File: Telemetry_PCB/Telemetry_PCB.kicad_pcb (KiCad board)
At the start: 2 copper layers, 11 parts, among them J1 Raspberry Pi Zero W, J2 Voltage Sensor, J3 Current Sensor, J4 ADC, J5 GPS

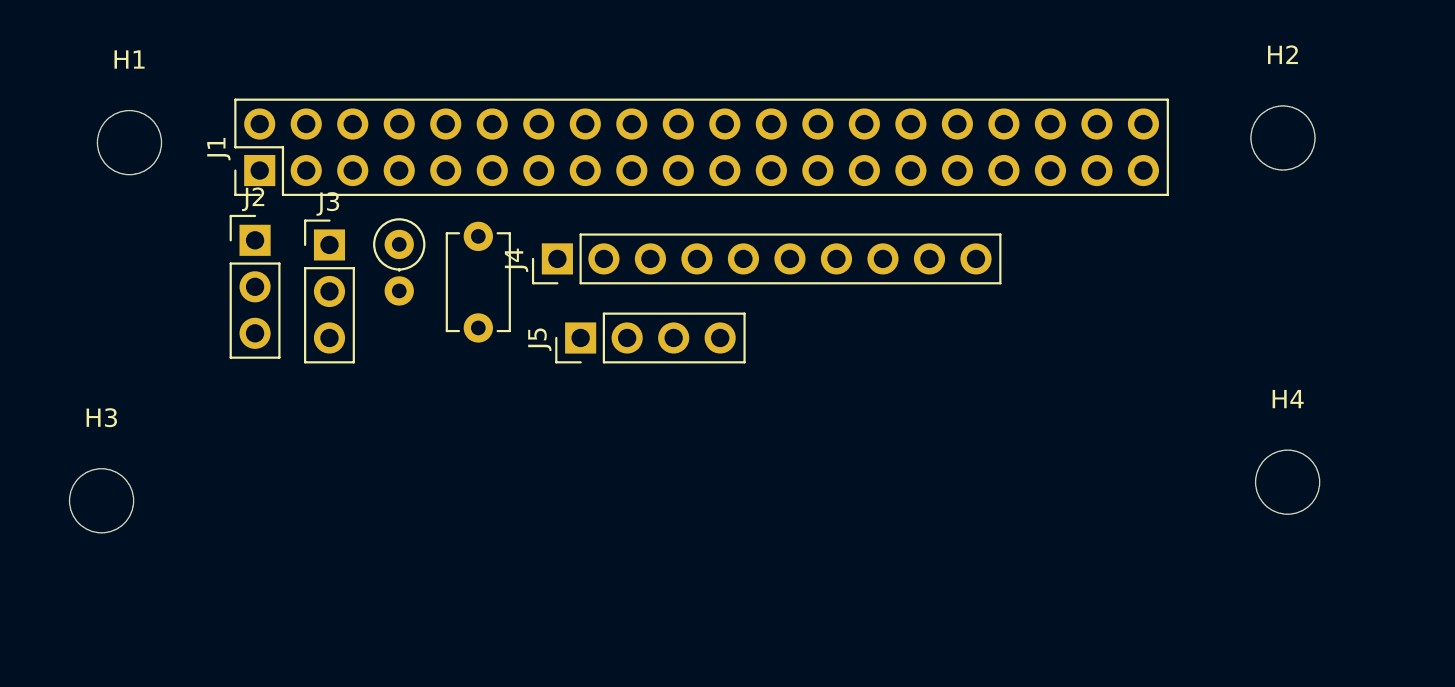
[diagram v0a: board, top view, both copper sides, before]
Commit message: Adding email system
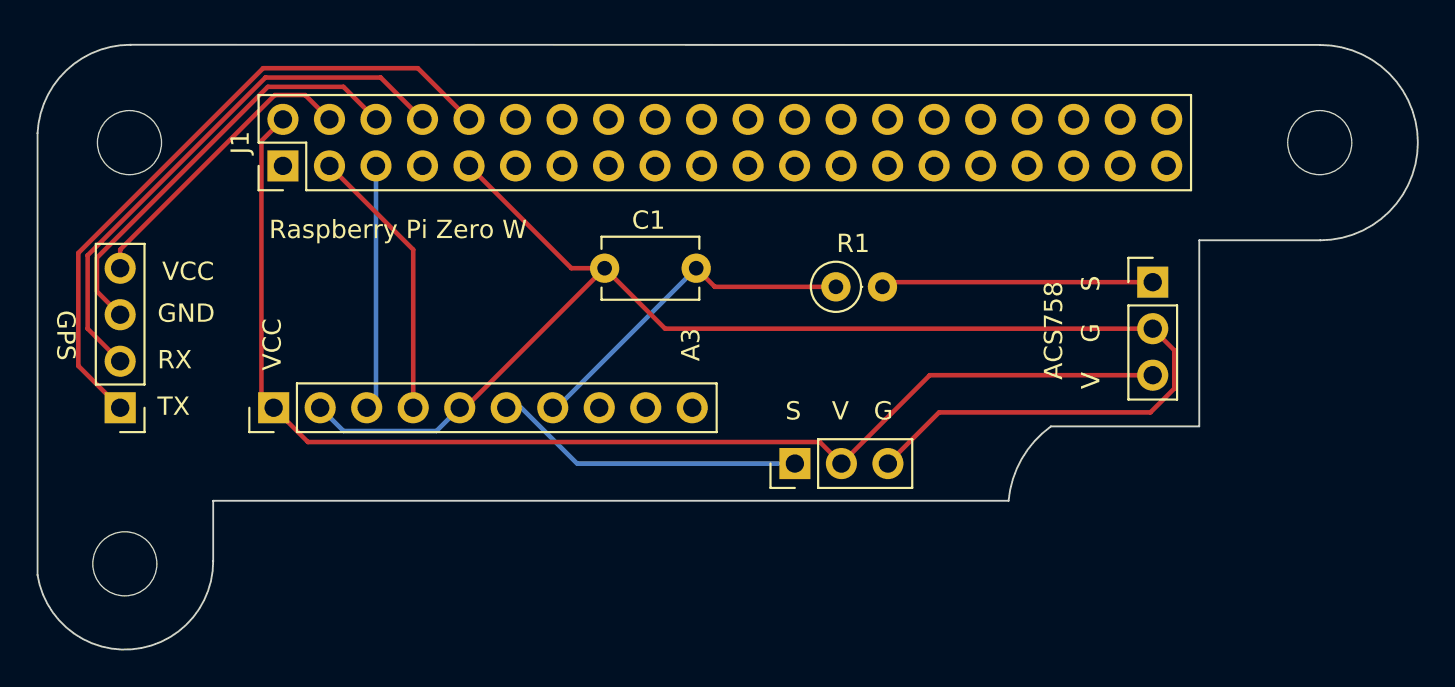
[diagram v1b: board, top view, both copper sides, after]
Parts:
- removed H4: MountingHole, MountingHole:MountingHole_3.5mm
- moved J3 45.0 mm to (157.5, 66.5)
- moved J2 31.9 mm to (137.9, 76.5), turned to 90 degrees
- moved J5 25.4 mm to (101.1, 73.4), turned to 180 degrees
- moved R1 24.0 mm to (140.2, 66.8), turned to 0 degrees
- moved J4 17.5 mm to (109.5, 73.4)
- moved C1 7.63 mm to (127.5, 65.8), turned to 0 degrees
- moved H3 3.67 mm to (101.3, 81.9)
- moved H2 2.02 mm to (166.6, 58.9)
- moved J1 1.30 mm to (110.0, 60.2)
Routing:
- net Net-(J1-Pin_9): track 0.00 -> 81.9 mm
- net Net-(J1-Pin_2): track 0.00 -> 67.8 mm
- net Net-(J1-Pin_10): track 0.00 -> 36.1 mm
- net Net-(J1-Pin_8): track 0.00 -> 29.8 mm
- net Net-(J1-Pin_6): track 0.00 -> 23.5 mm
- net Net-(J4-Pin_7): track 0.00 -> 19.0 mm
- net Net-(J2-Pin_1): track 0.00 -> 17.0 mm
- net Net-(J1-Pin_4): track 0.00 -> 16.5 mm
- net Net-(J3-Pin_1): track 0.00 -> 15.2 mm
- net Net-(J1-Pin_3): track 0.00 -> 15.1 mm
- net Net-(J1-Pin_5): track 0.00 -> 13.4 mm
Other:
- board outline added: 75.4 x 33 mm
- board text added: "A3"
- board text added: "ACS758"
- board text added: "C1"
- board text added: "G"
- board text added: "GND"
- board text added: "GPS"
- board text added: "R1"
- board text added: "RX"
- board text added: "Raspberry Pi Zero W"
- board text added: "S"
- board text added: "TX"
- board text added: "UMASS AERONAUTICS TELEMETRY 2023-2024"
- board text added: "V"
- board text added: "VCC"
